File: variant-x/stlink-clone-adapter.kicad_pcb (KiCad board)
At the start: 2 copper layers, 25.1 x 18 mm, 8 parts, among them J1 Conn_01x04, J2 Conn_01x04, J3 Conn_02x05_Odd_Even, J4 Conn_01x04, J5 Conn_ARM_JTAG_SWD_10

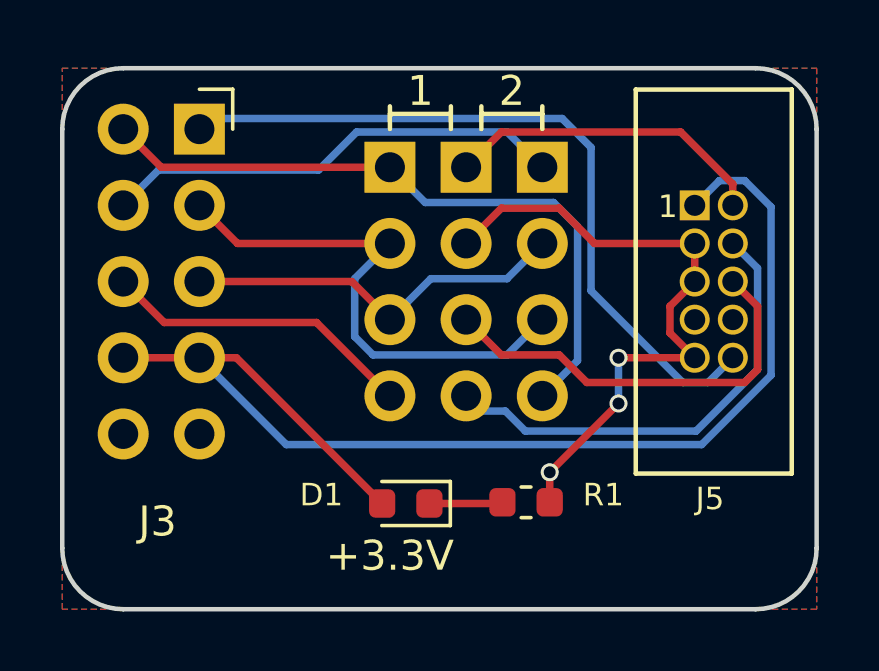
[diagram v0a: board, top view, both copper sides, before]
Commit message: try out fillets
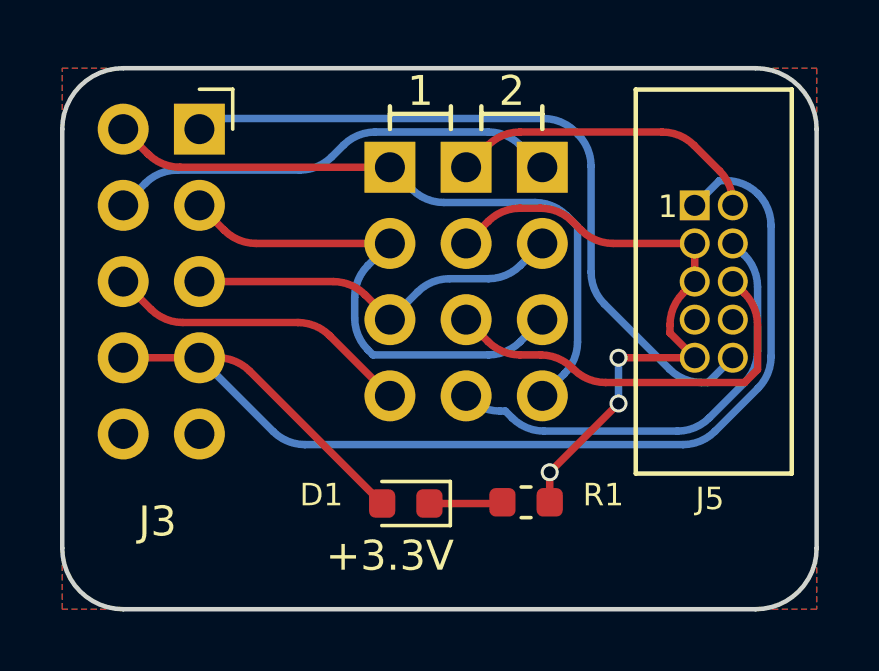
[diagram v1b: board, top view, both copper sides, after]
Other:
- net class Default removed
